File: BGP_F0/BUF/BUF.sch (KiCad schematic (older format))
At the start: 34 parts, among them P1 CONN_01X02, P2 CONN_01X02, P3 CONN_01X03, P4 CONN_01X02, P5 CONN_01X09, P6 CONN_01X05, P7 CONN_01X02, Q1 2N5457, Q2 2N5457, U1 MC33178

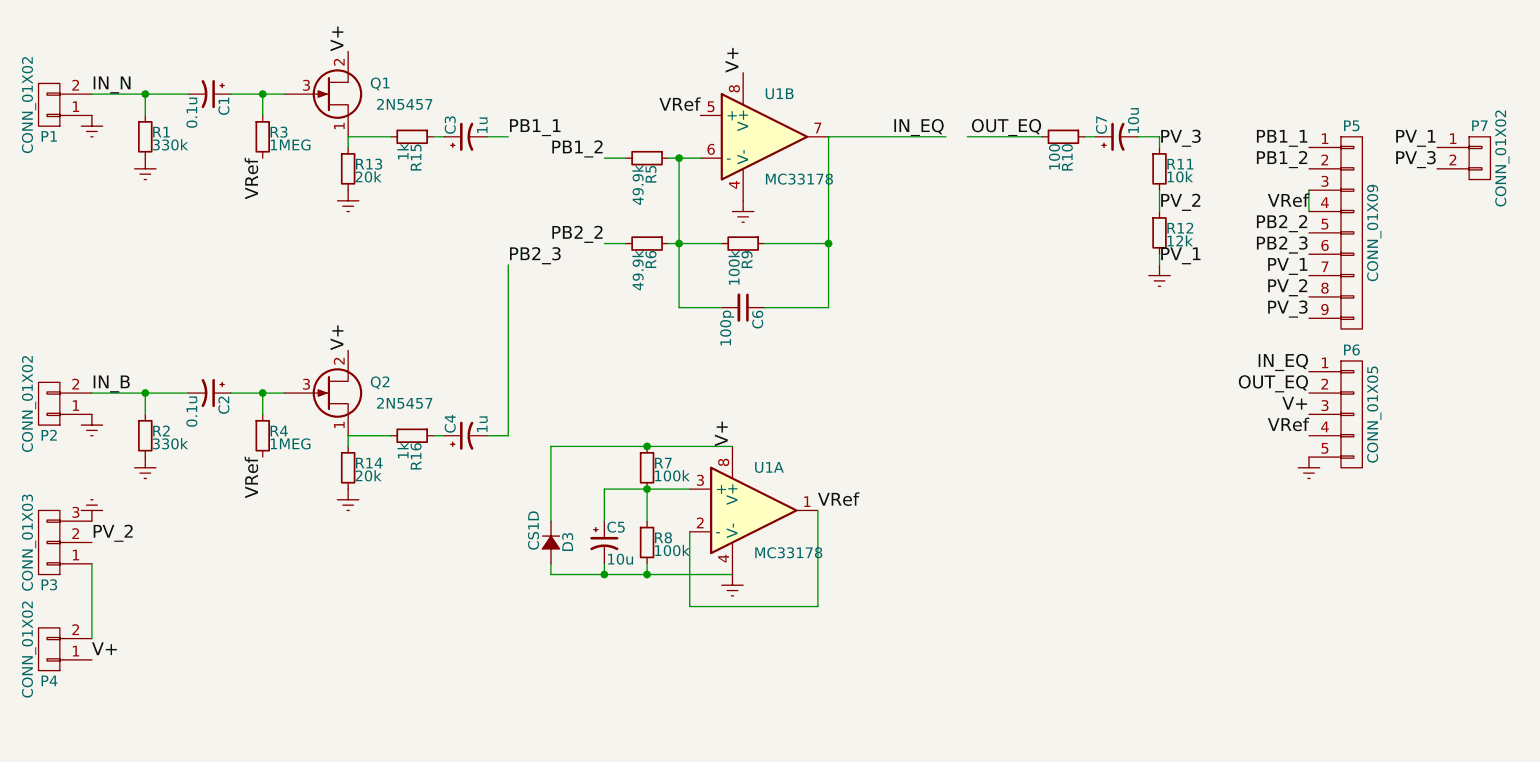
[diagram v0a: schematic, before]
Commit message: Some fixes and refinement
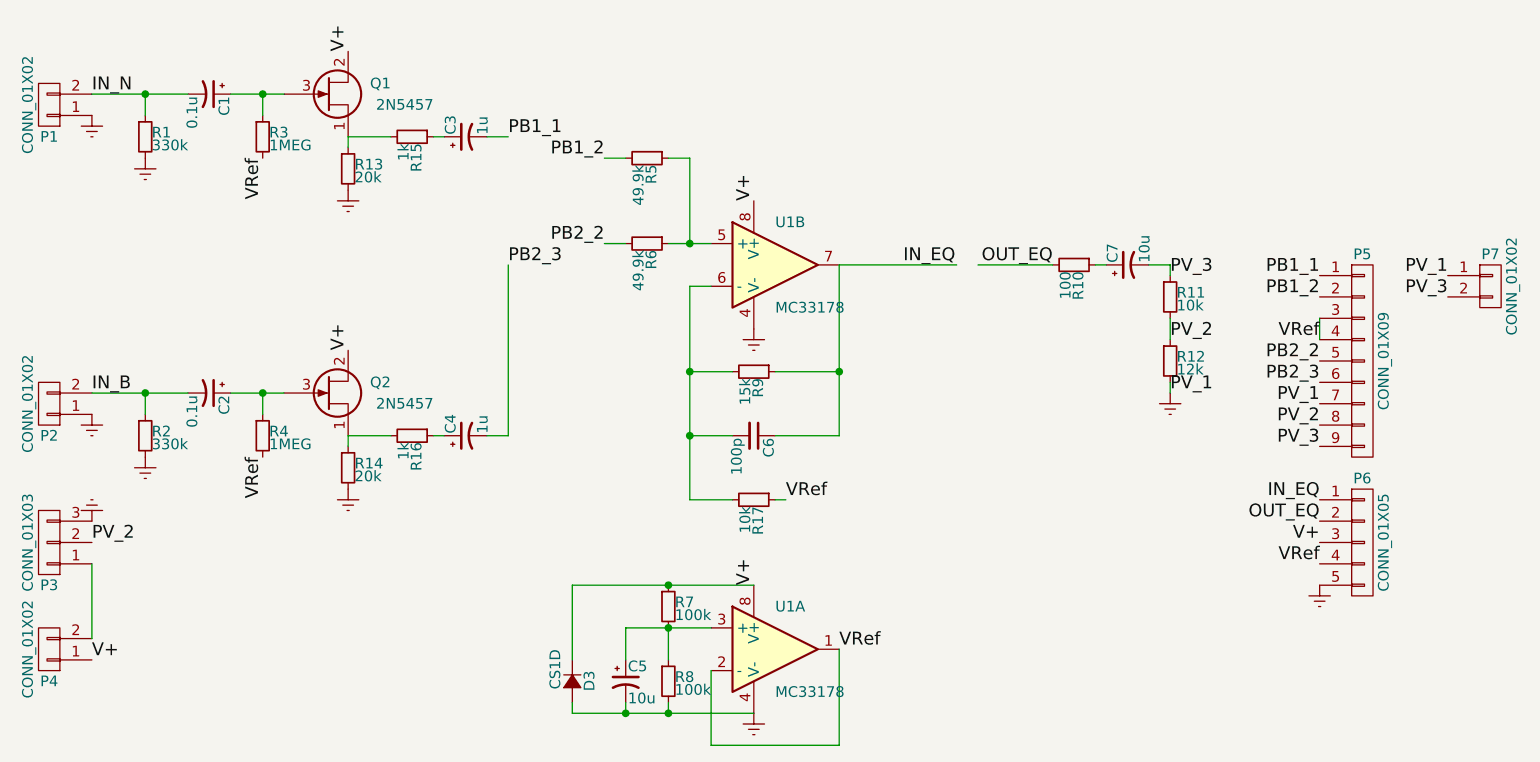
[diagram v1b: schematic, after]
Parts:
- added R17: 10k, Resistors_SMD:R_0603, symbol R_Small
- R9: value 100k -> 15k
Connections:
- wire segments 47 -> 52
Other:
- moved on the sheet: C5, C6, C7, D3, P5, P6, P7, R10, R11, R12, R7, R8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
